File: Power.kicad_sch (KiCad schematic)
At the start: 1 part, among them U2 Compute_Module_4_Functional

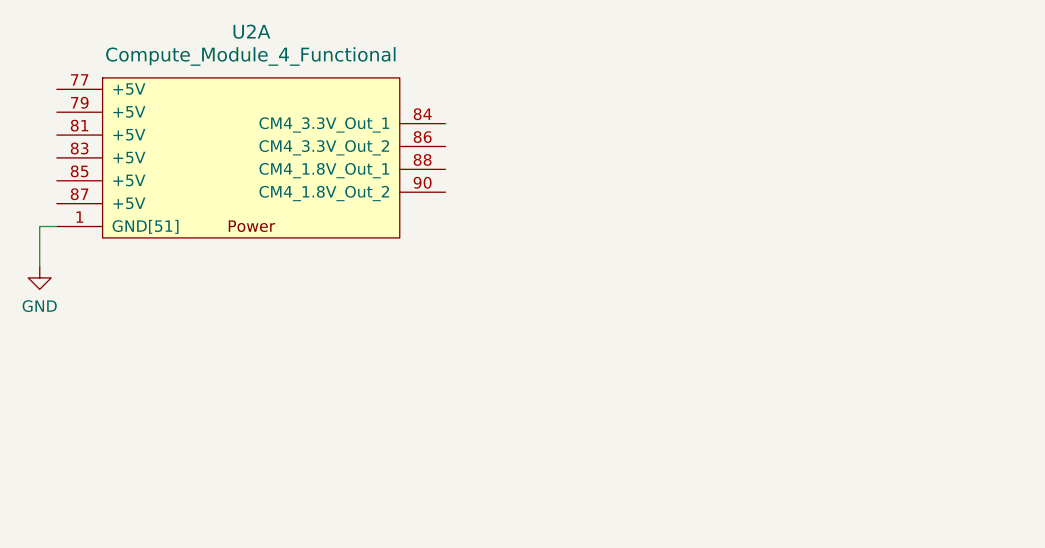
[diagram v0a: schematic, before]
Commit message: added display things + others
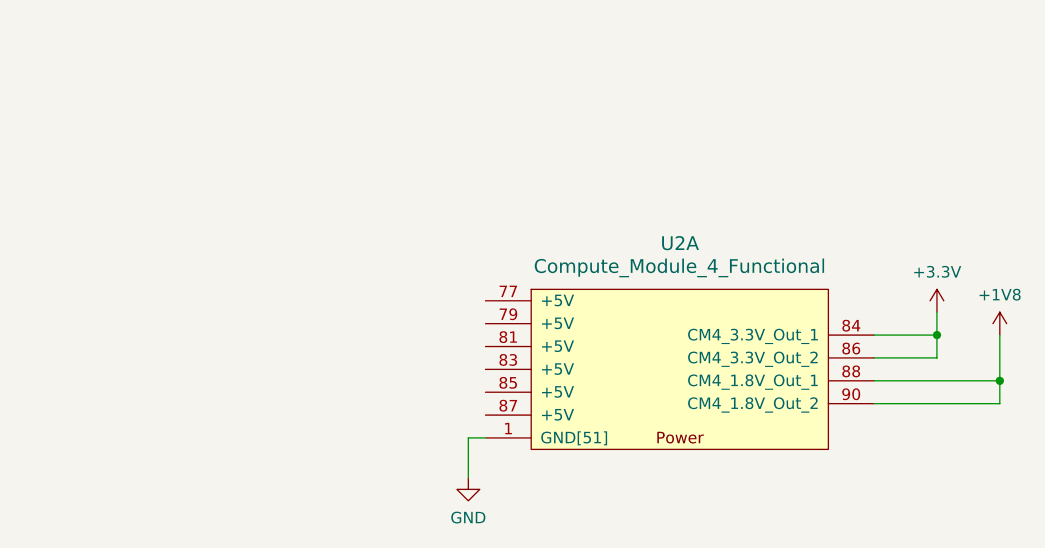
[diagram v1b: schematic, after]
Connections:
- net +3.3V: now reaches U2.84 (CM4_3.3V_Out_1)
- net +3.3V: now also U2.86 (CM4_3.3V_Out_2)
- net +1V8: now reaches U2.88 (CM4_1.8V_Out_1)
- net +1V8: now also U2.90 (CM4_1.8V_Out_2)
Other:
- moved on the sheet: U2A
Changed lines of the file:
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@@
 (kicad_sch (version 20230121) (generator eeschema)
   (paper "A4")
-  (wire (pts (xy 45.085 69.85) (xy 43.18 69.85))
-    (stroke (width 0) (type default))
-  )
-  (wire (pts (xy 43.18 69.85) (xy 43.18 74.295))
-    (stroke (width 0) (type default))
-  )
-  (symbol (lib_id "Raspberry_Pi_Compute_Module_4:Compute_Module_4_Functional") (at 45.085 55.88 0) (unit 1)
+  (junction (at 142.875 81.915) (diameter 0) (color 0 0 0 0)
+  )
+  (junction (at 149.86 86.995) (diameter 0) (color 0 0 0 0)
+  )
+  (wire (pts (xy 142.875 81.915) (xy 142.875 84.455))
+    (stroke (width 0) (type default))
+  )
+  (wire (pts (xy 149.86 86.995) (xy 149.86 89.535))
+    (stroke (width 0) (type default))
+  )
+  (wire (pts (xy 142.875 84.455) (xy 135.89 84.455))
+    (stroke (width 0) (type default))
+  )
+  (wire (pts (xy 149.86 81.915) (xy 149.86 86.995))
+    (stroke (width 0) (type default))
+  )
+  (wire (pts (xy 142.875 79.375) (xy 142.875 81.915))
+    (stroke (width 0) (type default))
+  )
+  (wire (pts (xy 92.71 93.345) (xy 90.805 93.345))
+    (stroke (width 0) (type default))
+  )
+  (wire (pts (xy 149.86 89.535) (xy 135.89 89.535))
+    (stroke (width 0) (type default))
+  )
+  (wire (pts (xy 90.805 93.345) (xy 90.805 97.79))
+    (stroke (width 0) (type default))
+  )
+  (wire (pts (xy 135.89 81.915) (xy 142.875 81.915))
+    (stroke (width 0) (type default))
+  )
+  (wire (pts (xy 135.89 86.995) (xy 149.86 86.995))
+    (stroke (width 0) (type default))
+  )
+  (symbol (lib_id "power:+1V8") (at 149.86 81.915 0) (unit 1)
     (in_bom yes) (on_board yes) (dnp no) (fields_autoplaced)
-    (property "Reference" "U2" (at 66.675 48.26 0)
+    (property "Reference" "#PWR017" (at 149.86 85.725 0)
+      (effects (font (size 1.27 1.27)) hide)
+    )
+    (property "Value" "+1V8" (at 149.86 77.47 0)
+      (effects (font (size 1.27 1.27)))
+    )
+    (property "Footprint" "" (at 149.86 81.915 0)
+      (effects (font (size 1.27 1.27)) hide)
+    )
+    (property "Datasheet" "" (at 149.86 81.915 0)
+      (effects (font (size 1.27 1.27)) hide)
+    )
+    (pin "1")
+    (instances
+      (project "CM4Emulator"
+        (path "/92f12c34-c5d8-4b38-8279-d435b24941c6/1b56670e-1cdd-434c-b5e9-8d50d2242662"
+          (reference "#PWR017") (unit 1)
+        )
+      )
+    )
+  )
+  (symbol (lib_id "power:+3.3V") (at 142.875 79.375 0) (unit 1)
+    (in_bom yes) (on_board yes) (dnp no) (fields_autoplaced)
+    (property "Reference" "#PWR016" (at 142.875 83.185 0)
+      (effects (font (size 1.27 1.27)) hide)
+    )
+    (property "Value" "+3.3V" (at 142.875 74.93 0)
+      (effects (font (size 1.27 1.27)))
+    )
+    (property "Footprint" "" (at 142.875 79.375 0)
+      (effects (font (size 1.27 1.27)) hide)
+    )
+    (property "Datasheet" "" (at 142.875 79.375 0)
+      (effects (font (size 1.27 1.27)) hide)
+    )
+    (pin "1")
+    (instances
+      (project "CM4Emulator"
+        (path "/92f12c34-c5d8-4b38-8279-d435b24941c6/1b56670e-1cdd-434c-b5e9-8d50d2242662"
+          (reference "#PWR016") (unit 1)
+        )
+      )
+    )
+  )
+  (symbol (lib_id "Raspberry_Pi_Compute_Module_4:Compute_Module_4_Functional") (at 92.71 79.375 0) (unit 1)
+    (in_bom yes) (on_board yes) (dnp no) (fields_autoplaced)
+    (property "Reference" "U2" (at 114.3 71.755 0)
       (effects (font (size 1.524 1.524)))
     )
-    (property "Value" "Compute_Module_4_Functional" (at 66.675 50.8 0)
+    (property "Value" "Compute_Module_4_Functional" (at 114.3 74.295 0)
       (effects (font (size 1.524 1.524)))
     )
-    (property "Footprint" "RPi_Compute_Module_4:Raspberry-Pi-4-Compute-Module" (at 50.165 54.61 0)
+    (property "Footprint" "RPi_Compute_Module_4:Raspberry-Pi-4-Compute-Module" (at 97.79 78.105 0)
       (effects (font (size 1.524 1.524)) (justify left) hide)
     )
-    (property "Datasheet" "" (at 50.165 59.69 0)
+    (property "Datasheet" "" (at 97.79 83.185 0)
       (effects (font (size 1.524 1.524)) (justify left) hide)
     )
@@
     )
   )
-  (symbol (lib_id "power:GND") (at 43.18 74.295 0) (unit 1)
+  (symbol (lib_id "power:GND") (at 90.805 97.79 0) (unit 1)
     (in_bom yes) (on_board yes) (dnp no) (fields_autoplaced)
-    (property "Reference" "#PWR02" (at 43.18 80.645 0)
-      (effects (font (size 1.27 1.27)) hide)
-    )
-    (property "Value" "GND" (at 43.18 78.74 0)
+    (property "Reference" "#PWR02" (at 90.805 104.14 0)
+      (effects (font (size 1.27 1.27)) hide)
+    )
+    (property "Value" "GND" (at 90.805 102.235 0)
       (effects (font (size 1.27 1.27)))
     )
-    (property "Footprint" "" (at 43.18 74.295 0)
-      (effects (font (size 1.27 1.27)) hide)
-    )
-    (property "Datasheet" "" (at 43.18 74.295 0)
-      (effects (font (size 1.27 1.27)) hide)
-    )
+    (property "Footprint" "" (at 90.805 97.79 0)
+      (effects (font (size 1.27 1.27)) hide)
+    )
+    (property "Datasheet" "" (at 90.805 97.79 0)
+      (effects (font (size 1.27 1.27)) hide)
+    )

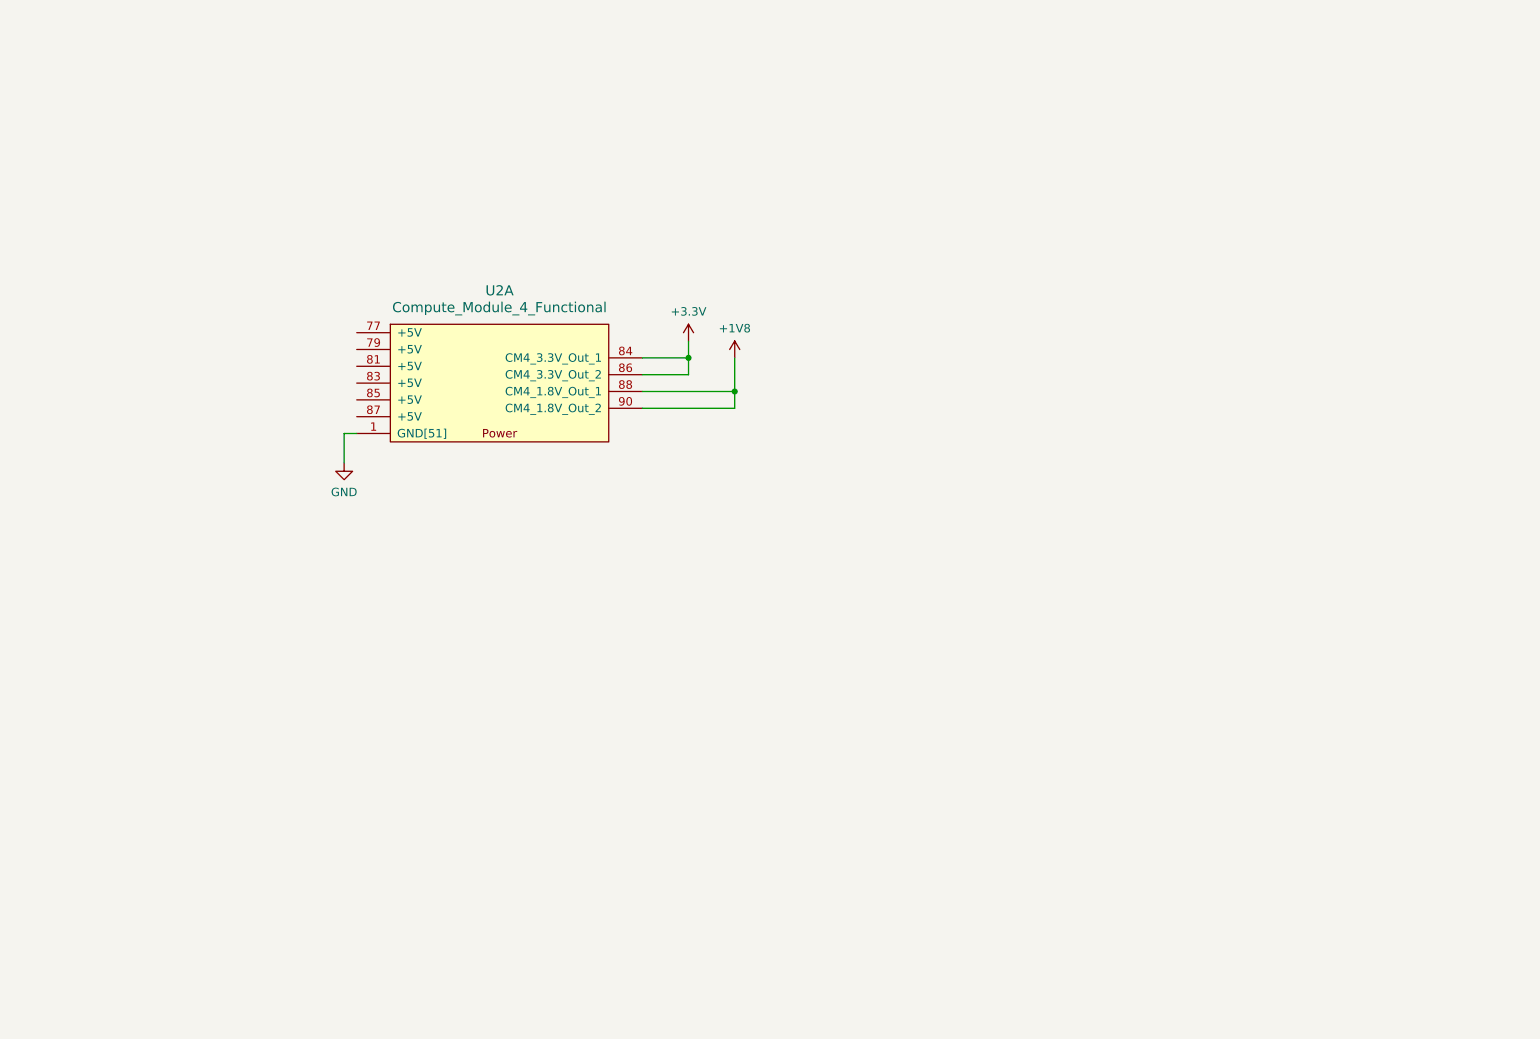
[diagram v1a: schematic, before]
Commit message: power changes
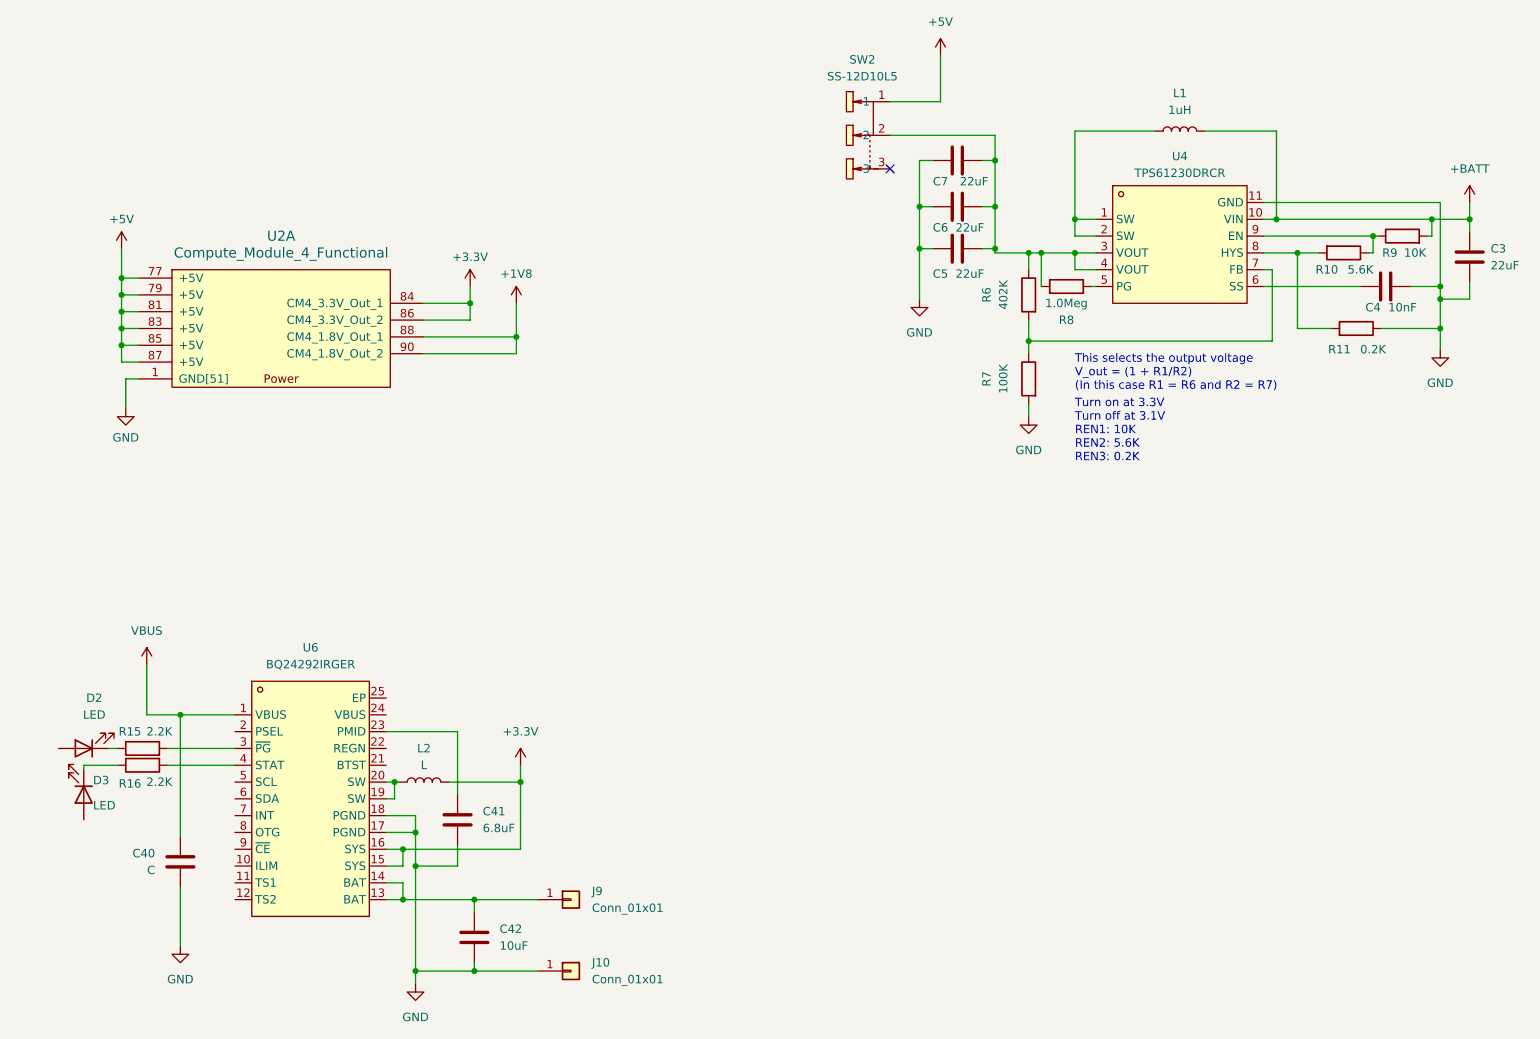
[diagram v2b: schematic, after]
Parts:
- added C3, C5, C6, C7: 22uF, Capacitor_SMD:C_0805_2012Metric, symbol Device:C
- added C4: 10nF, Capacitor_SMD:C_0402_1005Metric, symbol Device:C
- added C40: C, symbol Device:C
- added C41: 6.8uF, symbol Device:C
- added C42: 10uF, symbol Device:C
- added D2, D3: LED, symbol Device:LED
- added J10, J9: Conn_01x01, symbol Connector_Generic:Conn_01x01
- added L1: 1uH, Inductor_SMD:L_0603_1608Metric, symbol Device:L
- added L2: L, symbol Device:L
- added R10: 5.6K, Resistor_SMD:R_0603_1608Metric, symbol Device:R
- added R11: 0.2K, Resistor_SMD:R_0603_1608Metric, symbol Device:R
- added R15, R16: 2.2K, symbol Device:R
- added R6: 402K, Resistor_SMD:R_0603_1608Metric, symbol Device:R
- added R7: 100K, Resistor_SMD:R_0603_1608Metric, symbol Device:R
- added R8: 1.0Meg, Resistor_SMD:R_0603_1608Metric, symbol Device:R
- added R9: 10K, Resistor_SMD:R_0402_1005Metric, symbol Device:R
- added SW2: SS-12D10L5, easyeda2kicad:SW-TH_SS-12D10L5, symbol easyeda2kicad:SS-12D10L5
- added U4: TPS61230DRCR, easyeda2kicad:VSON-10_L3.0-W3.0-P0.50-TL-EP_TPS61230DRCR, symbol easyeda2kicad:TPS61230DRCR
- added U6: BQ24292IRGER, easyeda2kicad:QFN-24_L4.0-W4.0-P0.50-BL-EP2.7, symbol easyeda2kicad:BQ24292IRGER
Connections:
- net +3.3V: now also L2.2, U6.15 (SYS), U6.16 (SYS)
- net GND: now also C3.2, C4.2, C40.2, C41.2, C42.2, C5.1, C6.1, C7.1, J10.1 (Pin_1), R11.1, R7.2, U4.11 (GND), U6.17 (PGND), U6.18 (PGND)
- net +5V: now reaches U2.77 (+5V)
- net +5V: now also U2.79 (+5V), U2.81 (+5V), U2.83 (+5V), U2.85 (+5V), U2.87 (+5V), SW2.1
- new net: C42.1, J9.1 (Pin_1), U6.13 (BAT), U6.14 (BAT)
- new net: R8.1, U4.5 (PG)
- new net: C5.2, C6.2, C7.2, R6.1, R8.2, SW2.2, U4.3 (VOUT), U4.4 (VOUT)
- new net: L2.1, U6.19 (SW), U6.20 (SW)
- new net: D3.1 (K), R16.1
- new net: L1.1, U4.1 (SW), U4.2 (SW)
- new net: C4.1, U4.6 (SS)
- new net: R6.2, R7.1, U4.7 (FB)
- new net: R10.2, R11.2, U4.8 (HYS)
- new net: R10.1, R9.1, U4.9 (EN)
- new net: C41.1, U6.23 (PMID)
- new net: R15.2, U6.3 (~{PG})
- new net: R16.2, U6.4 (STAT)
- new net: D2.1 (K), R15.1
- new net +BATT: C3.1, L1.2, R9.2, U4.10 (VIN)
- new net VBUS: C40.1, U6.1 (VBUS)
- no-connect marks 0 -> 1
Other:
- note added: "This selects the output voltage V_out = (1 + R1/R2) (In this case R1 = R6 and R2 = R7)"
- note added: "Turn on at 3.3V Turn off at 3.1V REN1: 10K REN2: 5.6K REN3: 0.2K"
- moved on the sheet: U2A
